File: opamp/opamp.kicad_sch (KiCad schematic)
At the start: 8 parts, among them J1 Barrel_Jack, J2 AudioJack2, U1 ${SIM.PARAMS}

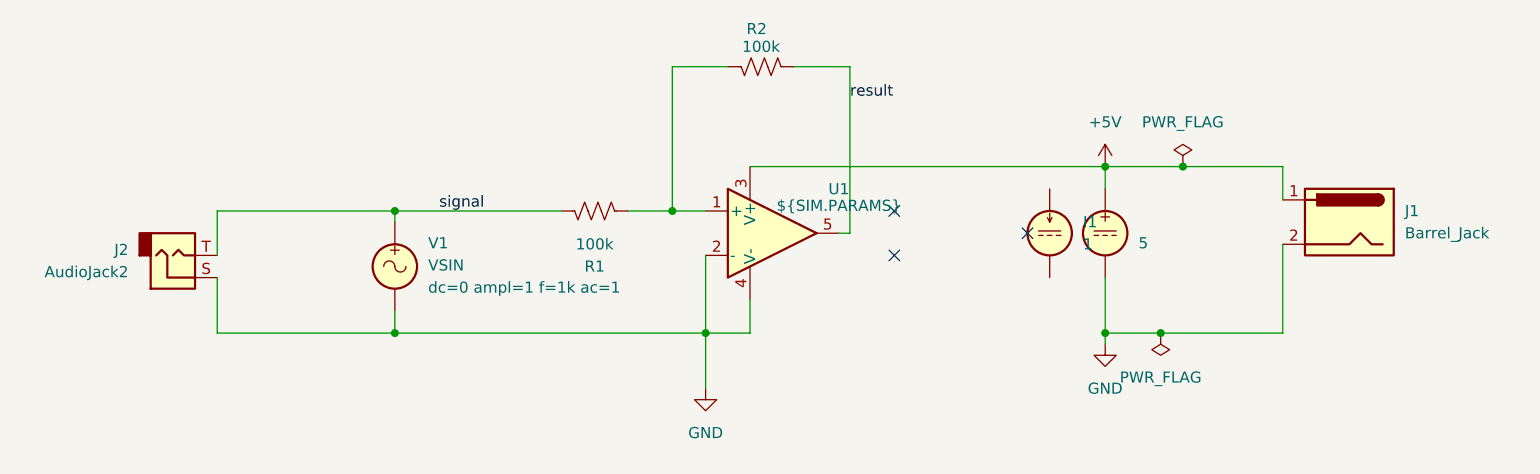
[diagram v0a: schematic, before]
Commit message: WIP
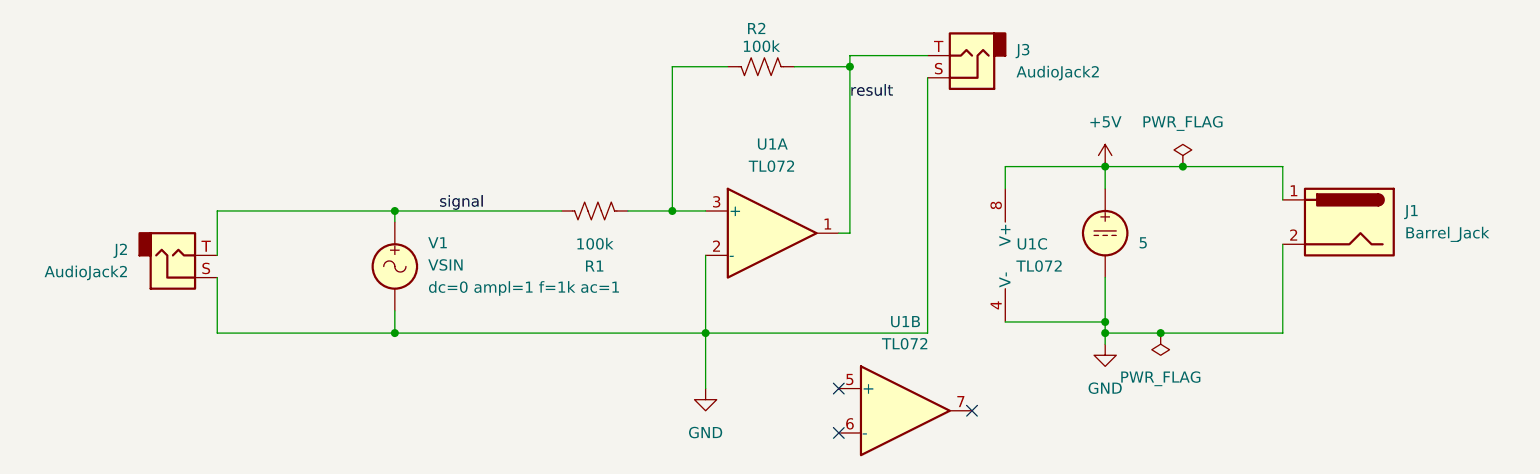
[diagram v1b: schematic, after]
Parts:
- removed I1: 1, symbol Simulation_SPICE:IDC
- removed U1: ${SIM.PARAMS}, symbol Simulation_SPICE:OPAMP
- added J3: AudioJack2, Connector_Audio:Jack_3.5mm_CUI_SJ1-3533NG_Horizontal_CircularHoles, symbol Connector_Audio:AudioJack2
- added U1: TL072, Package_DIP:DIP-8_W7.62mm, symbol Amplifier_Operational:TL072
- J1: footprint (none) -> Connector_BarrelJack:BarrelJack_Horizontal
- J2: footprint (none) -> Connector_Audio:Jack_3.5mm_CUI_SJ1-3533NG_Horizontal_CircularHoles
- R1, R2: footprint (none) -> Resistor_THT:R_Axial_DIN0207_L6.3mm_D2.5mm_P10.16mm_Horizontal
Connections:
- net +5V: now also U1.8 (V+)
- net GND: now also J3.S, U1.2 (-), U1.4 (V-)
- net result: now also J3.T, U1.1
- net at R1.2, R2.1: now also U1.3 (+)
